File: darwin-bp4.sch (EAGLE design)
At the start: 21 parts

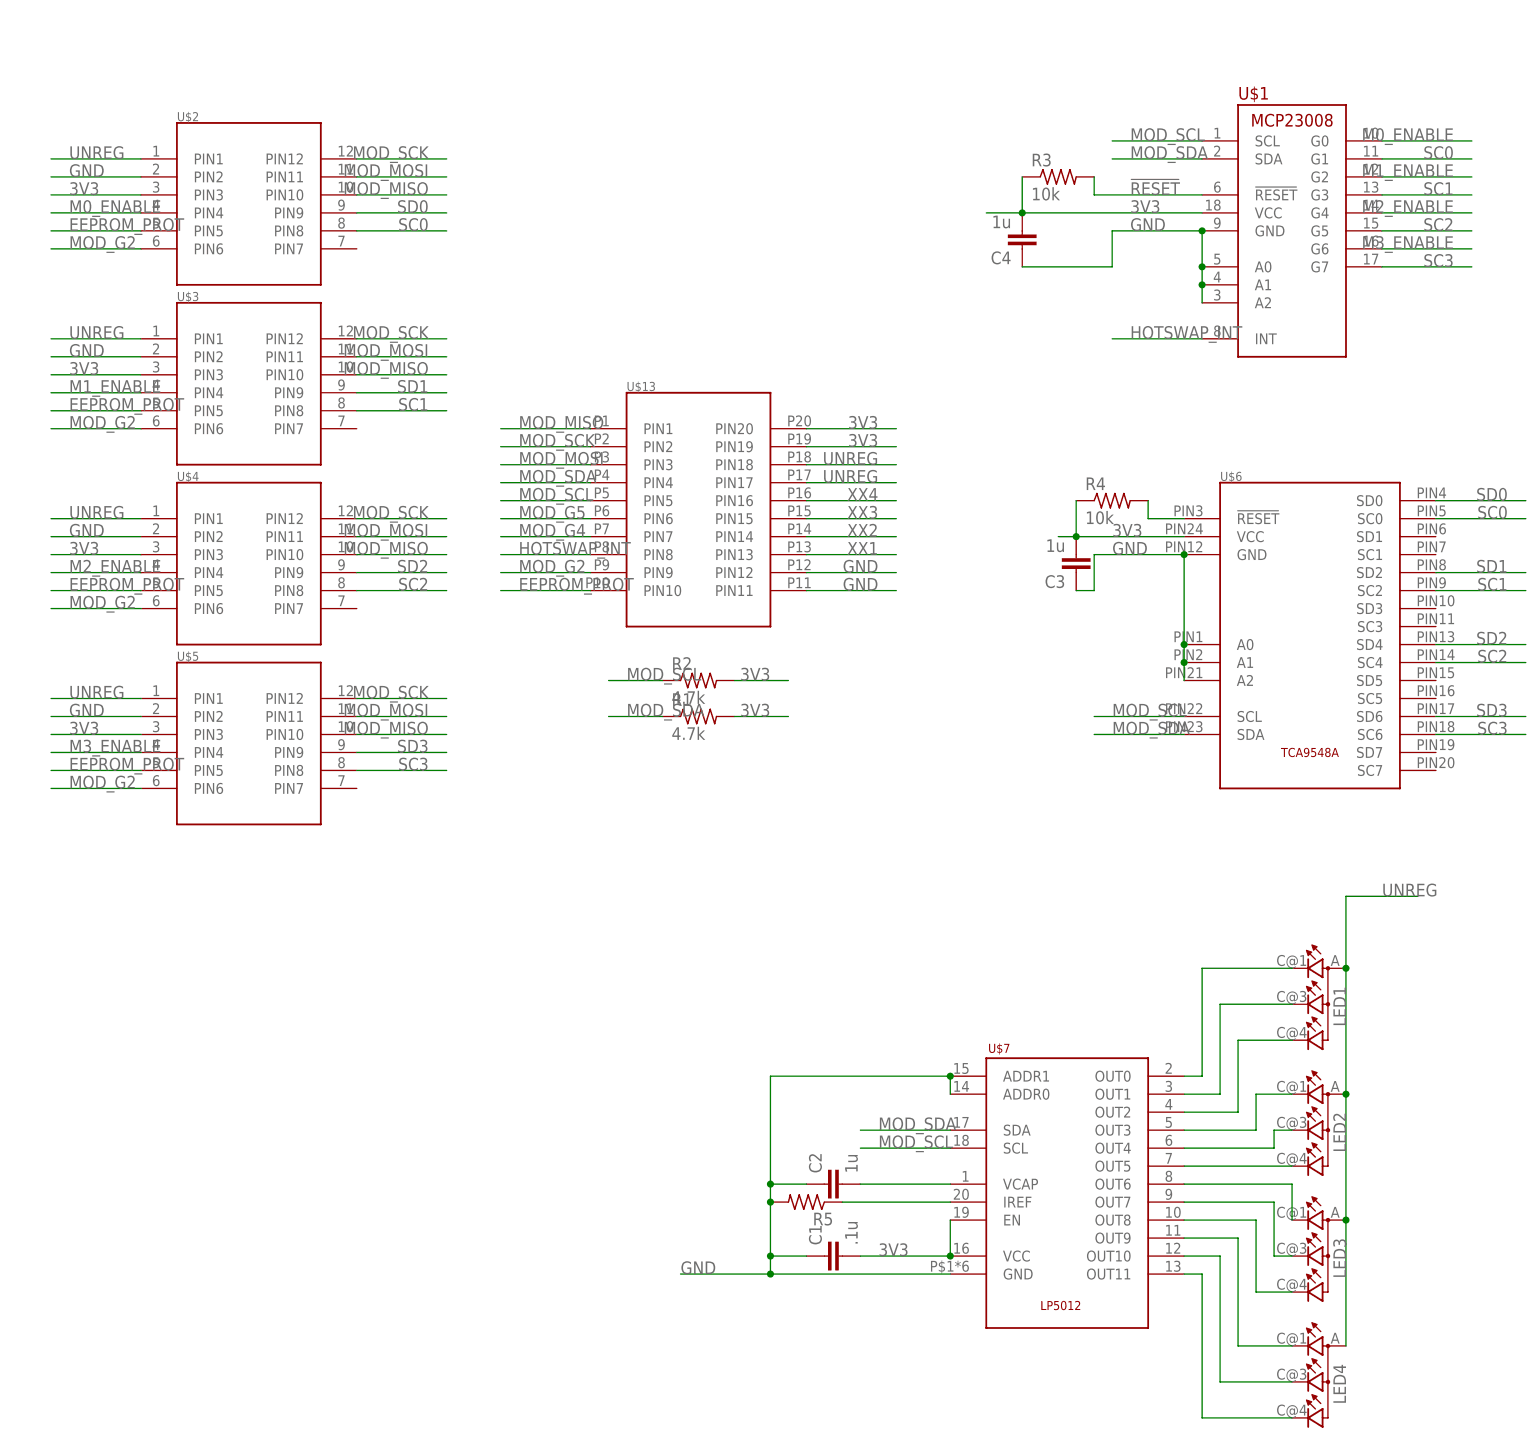
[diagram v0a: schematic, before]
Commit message: Cleanup.
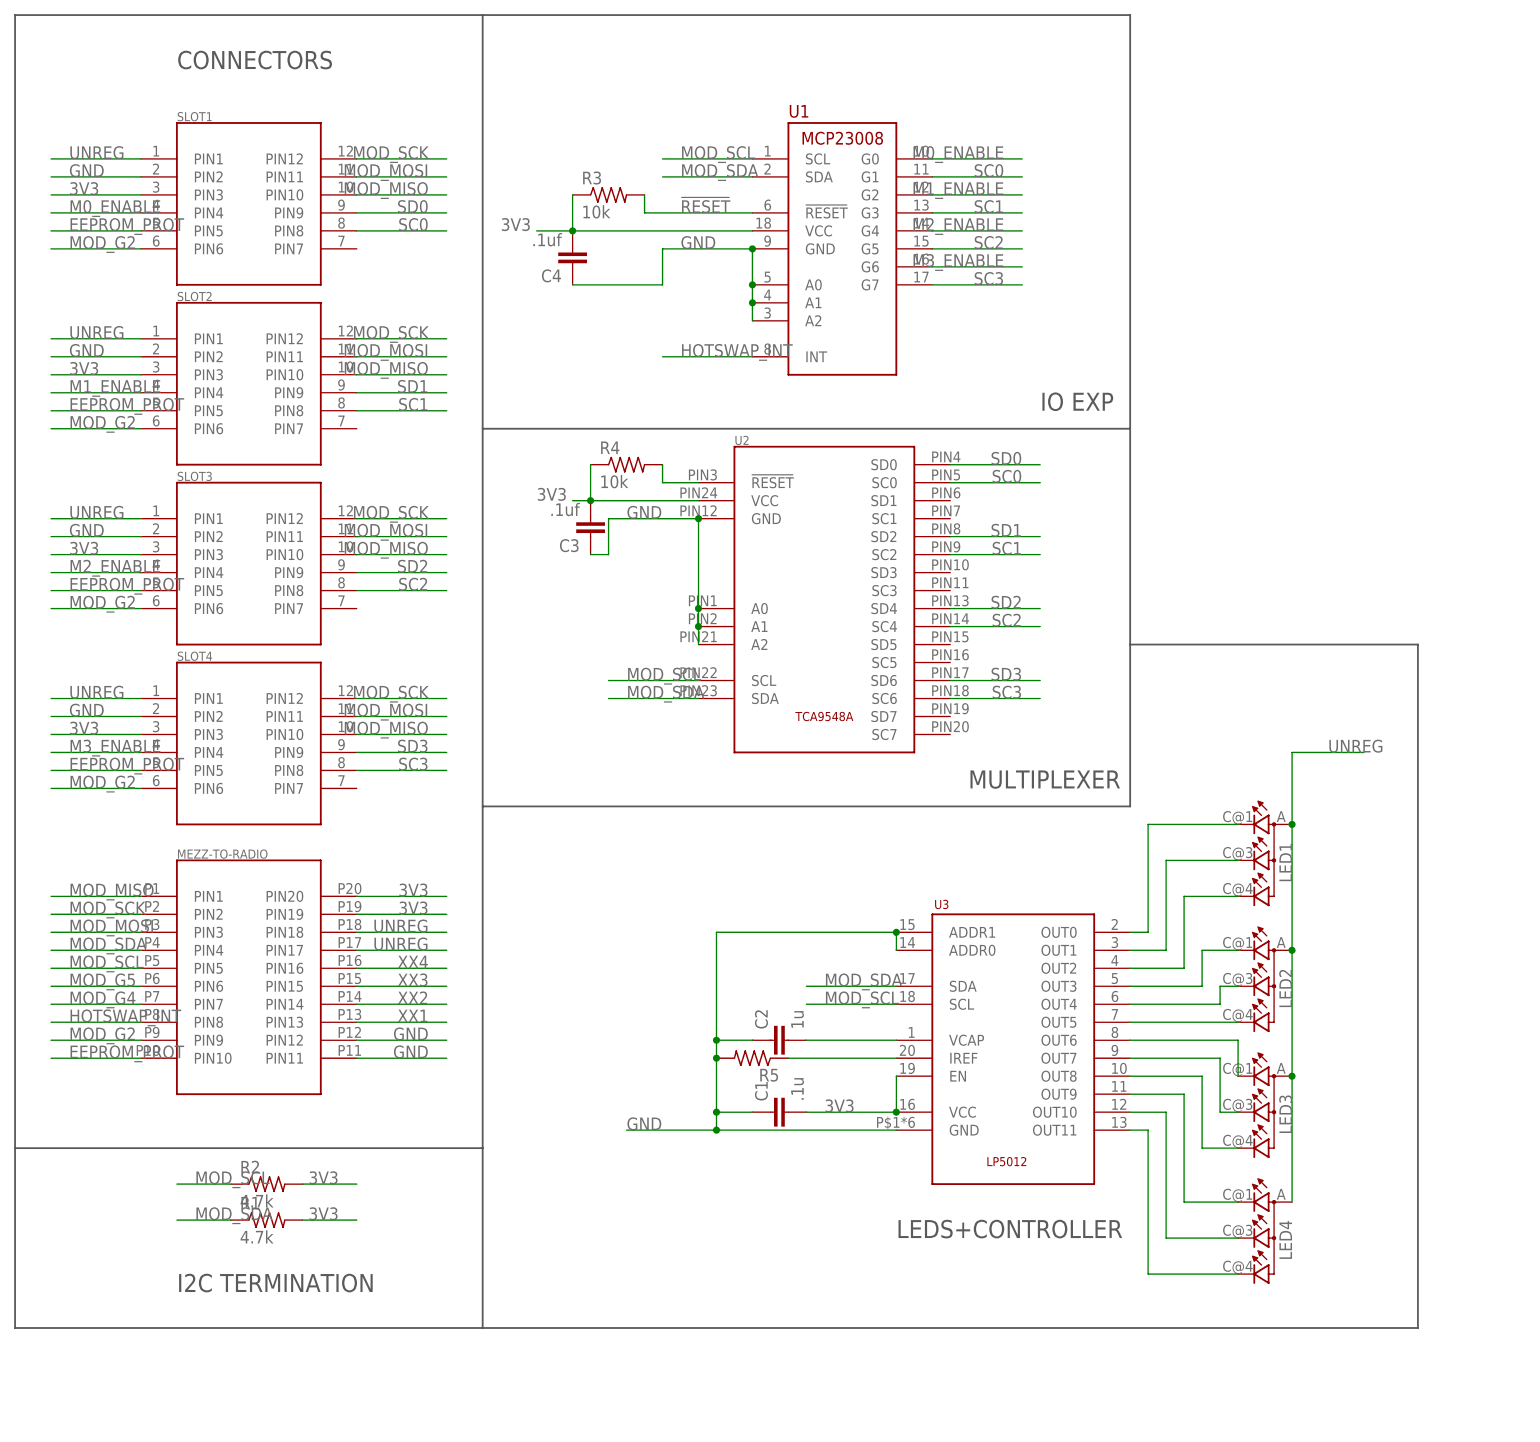
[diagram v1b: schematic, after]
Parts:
- removed U$1: MCP23008, Conservify:MCP23008
- removed U$13: M55-6102042R7102(M), Conservify:M55-6102042R7102(M)
- removed U$6: TCA9548A, Conservify:TCA9548A
- removed U$7: LP5012, Conservify:LP5012
- added MEZZ-TO-RADIO: M55-6102042R7102(M), Conservify:M55-6102042R7102(M)
- added U1: MCP23008, Conservify:MCP23008
- added U2: TCA9548A, Conservify:TCA9548A
- added U3: LP5012, Conservify:LP5012
- C3, C4: value 1u -> .1uf
- renumbered U$2 to SLOT1, U$3 to SLOT2, U$4 to SLOT3, U$5 to SLOT4
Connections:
- net !RESET: now also U1.!RESET; no longer U$1.!RESET
- net 3V3: now also MEZZ-TO-RADIO.PIN19, MEZZ-TO-RADIO.PIN20, U1.VCC, U2.VCC, U3.EN, U3.VCC; no longer U$1.VCC, U$13.PIN19, U$13.PIN20, U$6.VCC, U$7.EN, U$7.VCC
- net EEPROM_PROT: now also MEZZ-TO-RADIO.PIN10; no longer U$13.PIN10
- net GND: now also MEZZ-TO-RADIO.PIN11, MEZZ-TO-RADIO.PIN12, U1.A0, U1.A1, U1.A2, U1.GND, U2.A0, U2.A1, U2.A2, U2.GND, U3.ADDR0, U3.ADDR1, U3.GND; no longer U$1.A0, U$1.A1, U$1.A2, U$1.GND, U$13.PIN11, U$13.PIN12, U$6.A0, U$6.A1, U$6.A2, U$6.GND, U$7.ADDR0, U$7.ADDR1, U$7.GND
- net HOTSWAP_INT: now also MEZZ-TO-RADIO.PIN8, U1.INT; no longer U$1.INT, U$13.PIN8
- net M0_ENABLE: now also U1.G0; no longer U$1.G0
- net M1_ENABLE: now also U1.G2; no longer U$1.G2
- net M2_ENABLE: now also U1.G4; no longer U$1.G4
- net M3_ENABLE: now also U1.G6; no longer U$1.G6
- net MOD_G2: now also MEZZ-TO-RADIO.PIN9; no longer U$13.PIN9
- net MOD_G4: now also MEZZ-TO-RADIO.PIN7; no longer U$13.PIN7
- net MOD_G5: now also MEZZ-TO-RADIO.PIN6; no longer U$13.PIN6
- net MOD_MISO: now also MEZZ-TO-RADIO.PIN1; no longer U$13.PIN1
- net MOD_MOSI: now also MEZZ-TO-RADIO.PIN3; no longer U$13.PIN3
- net MOD_SCK: now also MEZZ-TO-RADIO.PIN2; no longer U$13.PIN2
- net MOD_SCL: now also MEZZ-TO-RADIO.PIN5, U1.SCL, U2.SCL, U3.SCL; no longer U$1.SCL, U$13.PIN5, U$6.SCL, U$7.SCL
- net MOD_SDA: now also MEZZ-TO-RADIO.PIN4, U1.SDA, U2.SDA, U3.SDA; no longer U$1.SDA, U$13.PIN4, U$6.SDA, U$7.SDA
- net N$1: now also U3.OUT0; no longer U$7.OUT0
- net N$11: now also U3.OUT8; no longer U$7.OUT8
- net N$12: now also U3.OUT9; no longer U$7.OUT9
- net N$13: now also U3.OUT10; no longer U$7.OUT10
- net N$14: now also U3.OUT11; no longer U$7.OUT11
- net N$2: now also U2.!RESET; no longer U$6.!RESET
- net N$20: now also U3.VCAP; no longer U$7.VCAP
- net N$21: now also U3.IREF; no longer U$7.IREF
- net N$3: now also U3.OUT1; no longer U$7.OUT1
- net N$4: now also U3.OUT2; no longer U$7.OUT2
- net N$5: now also U3.OUT3; no longer U$7.OUT3
- net N$6: now also U3.OUT4; no longer U$7.OUT4
- net N$7: now also U3.OUT5; no longer U$7.OUT5
- net N$8: now also U3.OUT6; no longer U$7.OUT6
- net N$9: now also U3.OUT7; no longer U$7.OUT7
- net SC0: now also U1.G1, U2.SC0; no longer U$1.G1, U$6.SC0
- net SC1: now also U1.G3, U2.SC2; no longer U$1.G3, U$6.SC2
- net SC2: now also U1.G5, U2.SC4; no longer U$1.G5, U$6.SC4
- net SC3: now also U1.G7, U2.SC6; no longer U$1.G7, U$6.SC6
- net SD0: now also U2.SD0; no longer U$6.SD0
- net SD1: now also U2.SD2; no longer U$6.SD2
- net SD2: now also U2.SD4; no longer U$6.SD4
- net SD3: now also U2.SD6; no longer U$6.SD6
- net UNREG: now also MEZZ-TO-RADIO.PIN17, MEZZ-TO-RADIO.PIN18; no longer U$13.PIN17, U$13.PIN18
- net XX1: now also MEZZ-TO-RADIO.PIN13; no longer U$13.PIN13
- net XX2: now also MEZZ-TO-RADIO.PIN14; no longer U$13.PIN14
- net XX3: now also MEZZ-TO-RADIO.PIN15; no longer U$13.PIN15
- net XX4: now also MEZZ-TO-RADIO.PIN16; no longer U$13.PIN16
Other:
- note added: "CONNECTORS"
- note added: "I2C TERMINATION"
- note added: "IO EXP"
- note added: "LEDS+CONTROLLER"
- note added: "MULTIPLEXER"
- moved on the sheet: C1, C2, C3, C4, LED1, LED2, LED3, LED4, R1, R2, R3, R4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
